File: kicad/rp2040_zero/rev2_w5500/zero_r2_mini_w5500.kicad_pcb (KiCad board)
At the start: 2 copper layers, 42.9 x 52.7 mm, 53 parts, among them J3 RP2040 Debug, J5 Debug port, P4 J1B1211CCD, Q1 DMG2302U, U1 RP2040-Zero, U5 W5500

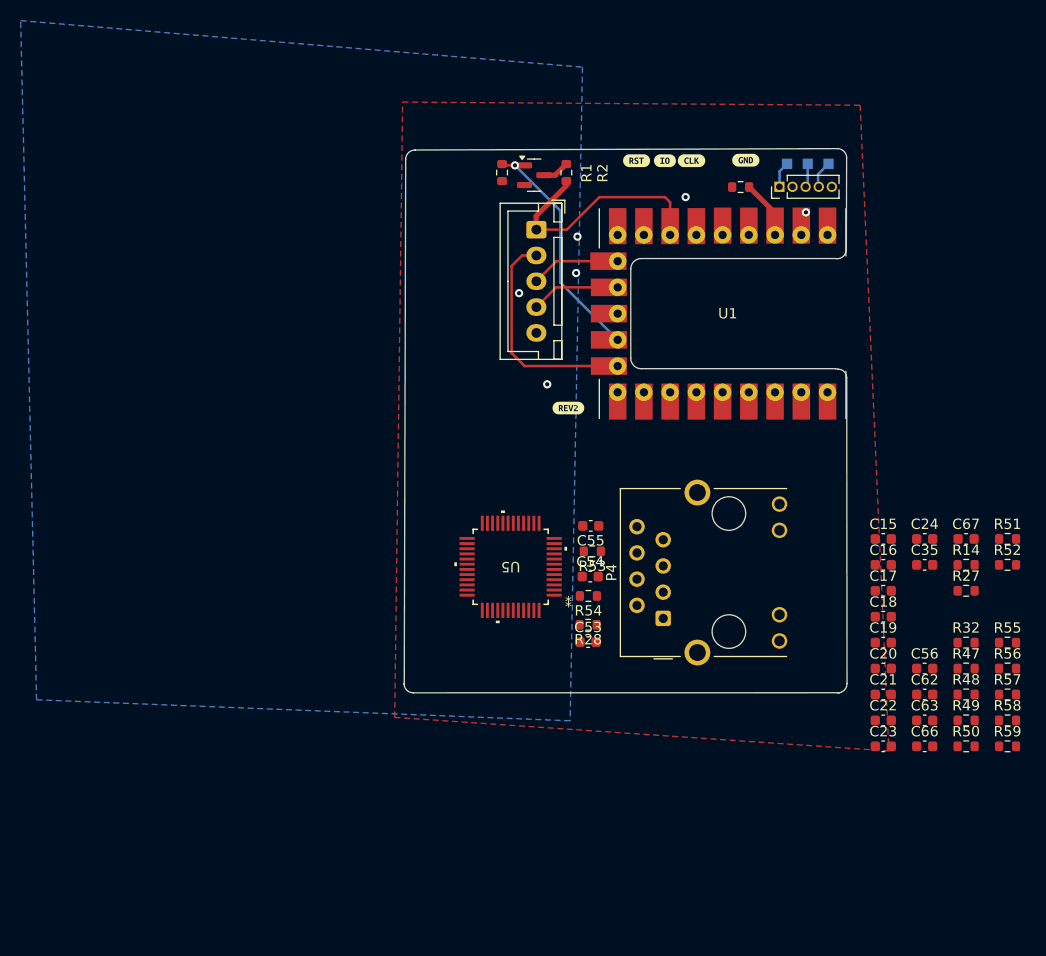
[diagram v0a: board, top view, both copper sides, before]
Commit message: w5500 : update 1
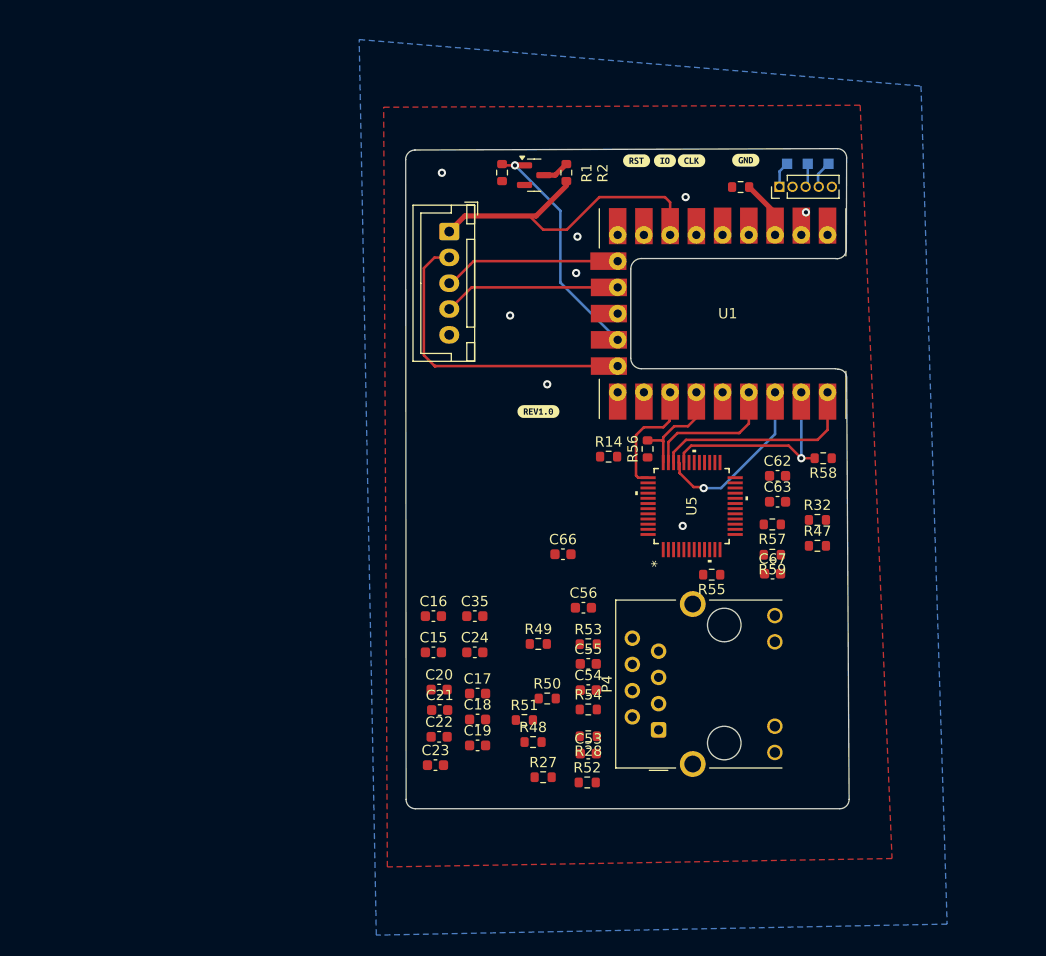
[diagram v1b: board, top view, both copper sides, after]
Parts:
- removed kibuzzard-6845954C: G***, kibuzzard-6845954C
- added kibuzzard-6A66F7EE: G***, kibuzzard-6A66F7EE, F.Cu at (120.3, 93.7)
- moved R51 50.0 mm to (118.9, 123.5)
- moved R52 45.8 mm to (125.0, 129.6)
- moved C15 44.9 mm to (110.1, 117.0)
- moved C24 44.9 mm to (114.1, 117.0)
- moved R27 44.8 mm to (120.7, 129.1)
- moved C16 43.8 mm to (110.1, 113.5)
- moved C35 43.8 mm to (114.1, 113.5)
- moved C23 43.4 mm to (110.3, 127.9)
- moved C20 43.1 mm to (110.6, 120.6)
- moved C22 43.0 mm to (110.6, 125.2)
- moved C21 43.0 mm to (110.7, 122.6)
- moved R48 42.2 mm to (119.7, 125.7)
- moved R49 42.1 mm to (120.2, 116.2)
- moved R56 40.8 mm to (130.8, 97.3), turned to 90 degrees
- moved R50 40.8 mm to (121.1, 121.4)
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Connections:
- R14 pad 1: /w5500b/RSTn -> RSTn
- R14 pad 2: 3V3 -> unconnected-(R14-Pad2)
- R32 pad 1: Net-(P4-GLED_K) -> LINKn
- R32 pad 2: /w5500b/LINKn -> Net-(P4-GLED_K)
- R47 pad 1: Net-(P4-YLED_K) -> ACTn
- R47 pad 2: /w5500b/ACTn -> Net-(P4-YLED_K)
- R56 pad 2: /w5500b/INTn -> INTn
- R58 pad 2: /w5500b/SPI0_CSn -> CSn
- U1 pad 10: unconnected-(U1-GP0-Pad10) -> MISO
- U1 pad 11: unconnected-(U1-GP1-Pad11) -> CSn
- U1 pad 12: unconnected-(U1-GP2-Pad12) -> CLK
- U1 pad 13: unconnected-(U1-GP3-Pad13) -> MOSI
- U1 pad 15: unconnected-(U1-GP5-Pad15) -> INTn
- U1 pad 16: unconnected-(U1-GP6-Pad16) -> RSTn
- U5 pad 25: /w5500b/LINKn -> LINKn
- U5 pad 27: /w5500b/ACTn -> ACTn
- U5 pad 32: /w5500b/SPI0_CSn -> CSn
- U5 pad 33: /w5500b/SPI0_SCK -> CLK
- U5 pad 34: /w5500b/SPI0_RX -> MISO
- U5 pad 35: /w5500b/SPI0_TX -> MOSI
- U5 pad 36: /w5500b/INTn -> INTn
- U5 pad 37: /w5500b/RSTn -> RSTn
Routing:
- net CSn: track 0.00 -> 20.8 mm, vias 0 -> 1
- net MISO: track 0.00 -> 19.5 mm
- net CLK: track 0.00 -> 17.3 mm, vias 0 -> 1
- net RSTn: track 0.00 -> 12.7 mm
- net MOSI: track 0.00 -> 12.6 mm
- net INTn: track 0.00 -> 9.56 mm
- net INOUT_NRESET: track 22.2 -> 31.2 mm
- net OUT_UART_RX: track 21.2 -> 29.8 mm
- net OUT_SWDCLK: track 7.81 -> 16.4 mm
- net OUT_SWDIO: track 8.68 -> 17.2 mm
- net GND: vias 6 -> 8
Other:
- board size 42.9 x 52.7 mm -> 42.9 x 63.9 mm

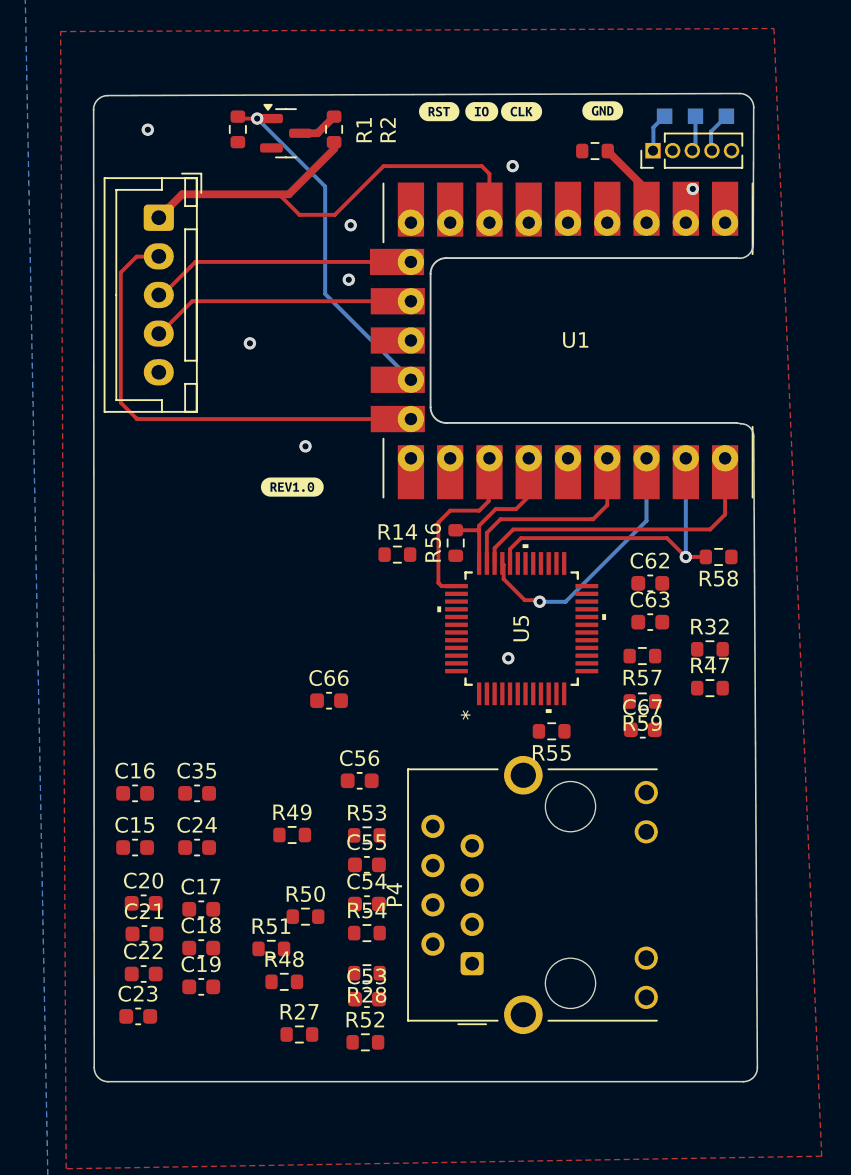
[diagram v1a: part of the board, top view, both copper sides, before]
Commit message: preliminary W5500
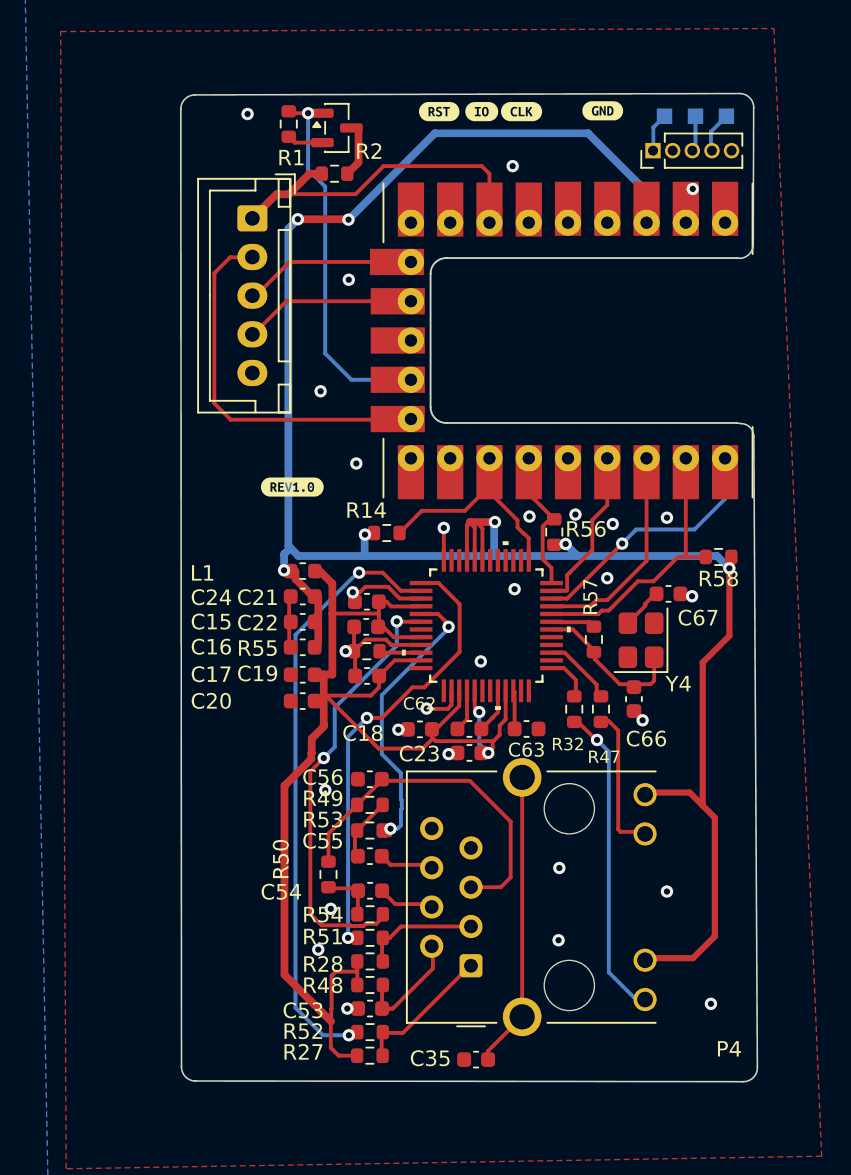
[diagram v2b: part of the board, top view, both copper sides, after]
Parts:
- removed C10: 100n, Resistor_SMD:R_0603_1608Metric
- removed R59: 0R, Resistor_SMD:R_0603_1608Metric
- added L1: HH-1M1608-121JT, Inductor_SMD:L_0603_1608Metric, F.Cu at (120.9, 99.1)
- added Y4: 25MHz, Crystal:Crystal_SMD_TXC_7M-4Pin_3.2x2.5mm, F.Cu at (142.8, 103.6)
- moved C23 27.4 mm to (131.7, 110.9)
- moved C22 26.7 mm to (125.0, 102.7)
- moved C21 25.9 mm to (125.1, 101.1)
- moved C35 24.9 mm to (132.1, 130.7)
- moved C19 22.8 mm to (125.1, 105.9)
- moved C18 20.0 mm to (128.5, 109.3)
- moved C66 19.7 mm to (142.4, 107.4), turned to 90 degrees
- moved C15 18.2 mm to (120.9, 102.4)
- moved C24 17.6 mm to (120.9, 100.7)
- moved C20 16.6 mm to (120.9, 107.5)
- moved C17 16.5 mm to (120.9, 105.8)
- moved C62 15.0 mm to (131.7, 109.3)
- moved C16 14.4 mm to (120.9, 104.0)
- moved R55 13.0 mm to (125.1, 104.3)
- moved C63 10.6 mm to (135.4, 109.3), turned to 180 degrees
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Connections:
- net INTn renamed W5INTn
- net RSTn renamed W5RSTn
- C15 pad 2: 3V3 -> +3.3V
- C16 pad 2: 3V3 -> +3.3V
- C24 pad 2: 3V3 -> +3.3V
- C35 pad 2: CHGND -> SH
- P4 pad 10: 3V3 -> +3.3V
- P4 pad 12: 3V3 -> +3.3V
- P4 pad SH: (no net) -> SH
- R14 pad 2: unconnected-(R14-Pad2) -> +3.3V
- R56 pad 1: 3V3 -> +3.3V
- R58 pad 1: 3V3 -> +3.3V
- U5 pad 28: 3V3 -> +3.3V
- U5 pad 43: 3V3 -> +3.3V
- U5 pad 44: 3V3 -> +3.3V
- U5 pad 45: 3V3 -> +3.3V
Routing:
- net +3.3V: track 3.55 -> 133.9 mm, vias 0 -> 7
- net 3V3A: track 0.00 -> 86.1 mm, vias 0 -> 2
- net Net-(U5-TXP): track 0.00 -> 38.6 mm, vias 0 -> 2
- net Net-(U5-TXN): track 0.00 -> 28.6 mm, vias 0 -> 2
- net Net-(U5-RXP): track 0.00 -> 28.1 mm, vias 0 -> 2
- net GND: track 0.00 -> 25.8 mm, vias 8 -> 29
- net Net-(P4-RCT): track 0.00 -> 22.7 mm
- net Net-(P4-GLED_K): track 0.00 -> 20.1 mm, vias 0 -> 1
- net SH: track 0.00 -> 19.2 mm
- net Net-(U5-RXN): track 0.00 -> 18.8 mm, vias 0 -> 2
- net /w5500b/XI: track 0.00 -> 9.55 mm
- net Net-(P4-YLED_K): track 0.00 -> 9.48 mm
- net Net-(P4-TD+): track 0.00 -> 9.38 mm
- net INOUT_NRESET: track 31.2 -> 21.9 mm
- net Net-(P4-TCT): track 0.00 -> 7.78 mm
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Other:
- board size 42.9 x 63.9 mm -> 37.3 x 63.9 mm
